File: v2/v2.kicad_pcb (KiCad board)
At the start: 2 copper layers, 9.7 x 8.4 mm, 97 parts, among them SW1 SW_Push, SW10 SW_Push, SW11 SW_Push, SW12 SW_Push, SW13 SW_Push, SW14 SW_Push, SW15 SW_Push, SW16 SW_Push, SW17 SW_Push, SW18 SW_Push, SW19 SW_Push, SW2 SW_Push, SW20 SW_Push, SW21 SW_Push, SW22 SW_Push, SW23 SW_Push, SW24 SW_Push, SW25 SW_Push, SW26 SW_Push, SW27 SW_Push, SW28 SW_Push, SW29 SW_Push, SW3 SW_Push, SW30 SW_Push, SW31 SW_Push, SW32 SW_Push, SW4 SW_Push, SW5 SW_Push, SW6 SW_Push, SW7 SW_Push, SW8 SW_Push, SW9 SW_Push, U1 Pico

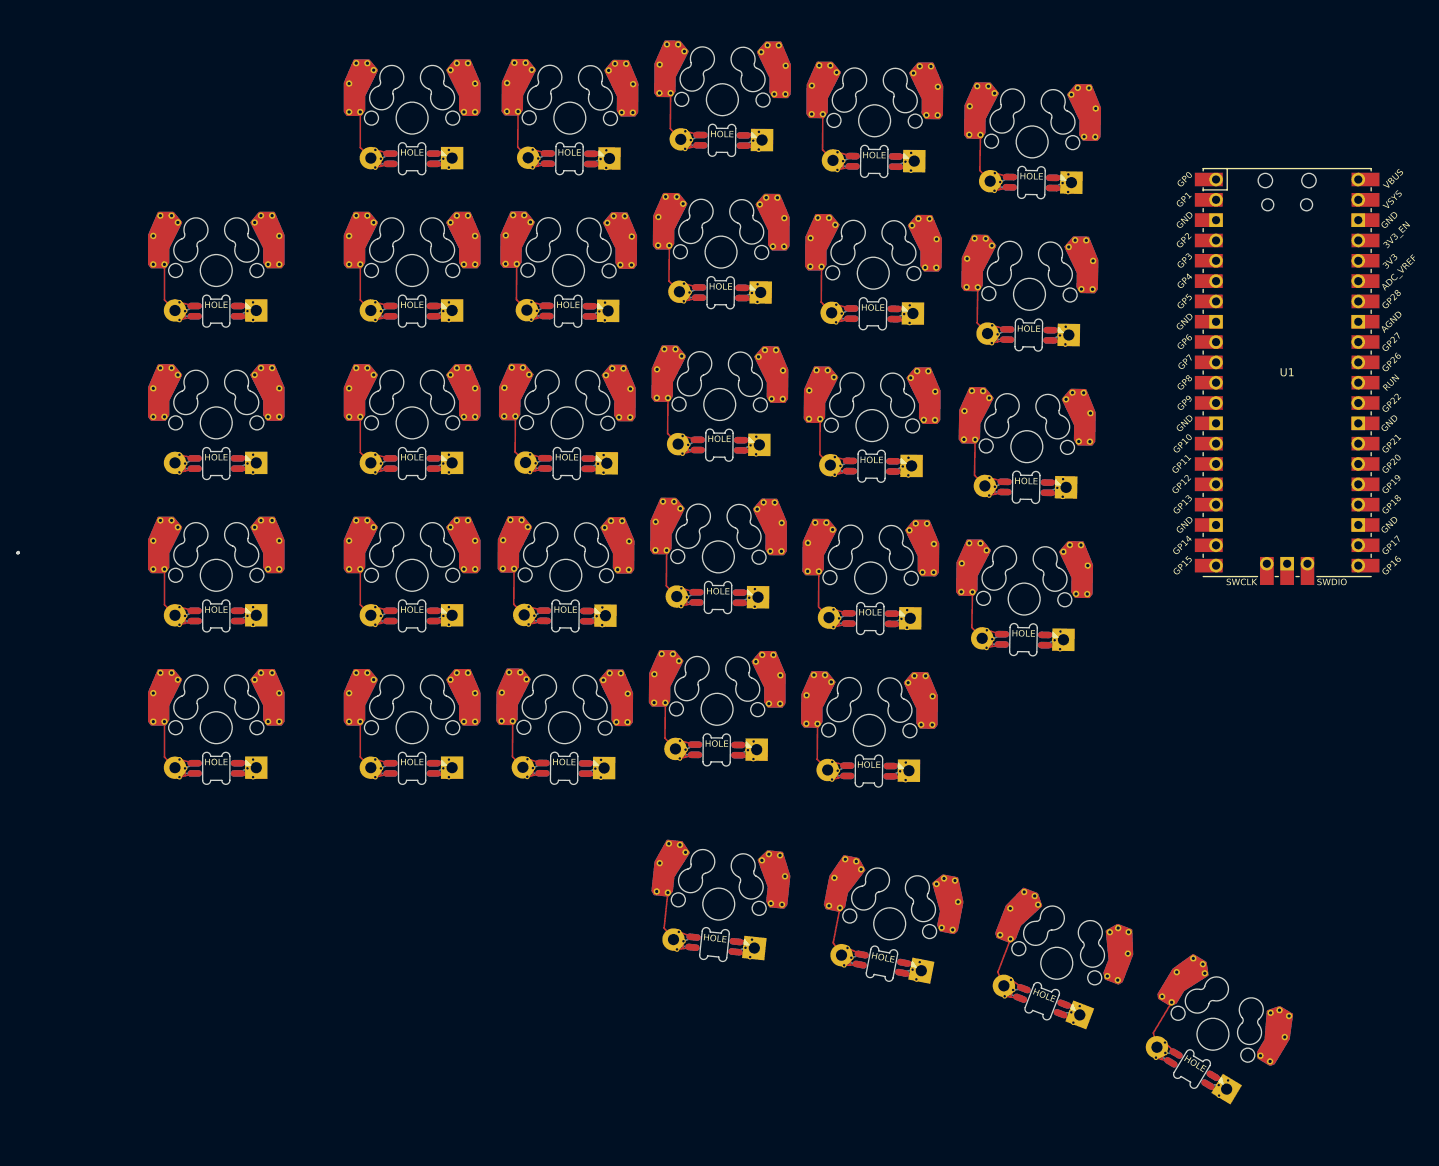
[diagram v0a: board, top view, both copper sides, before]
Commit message: schematic finished + some pcb
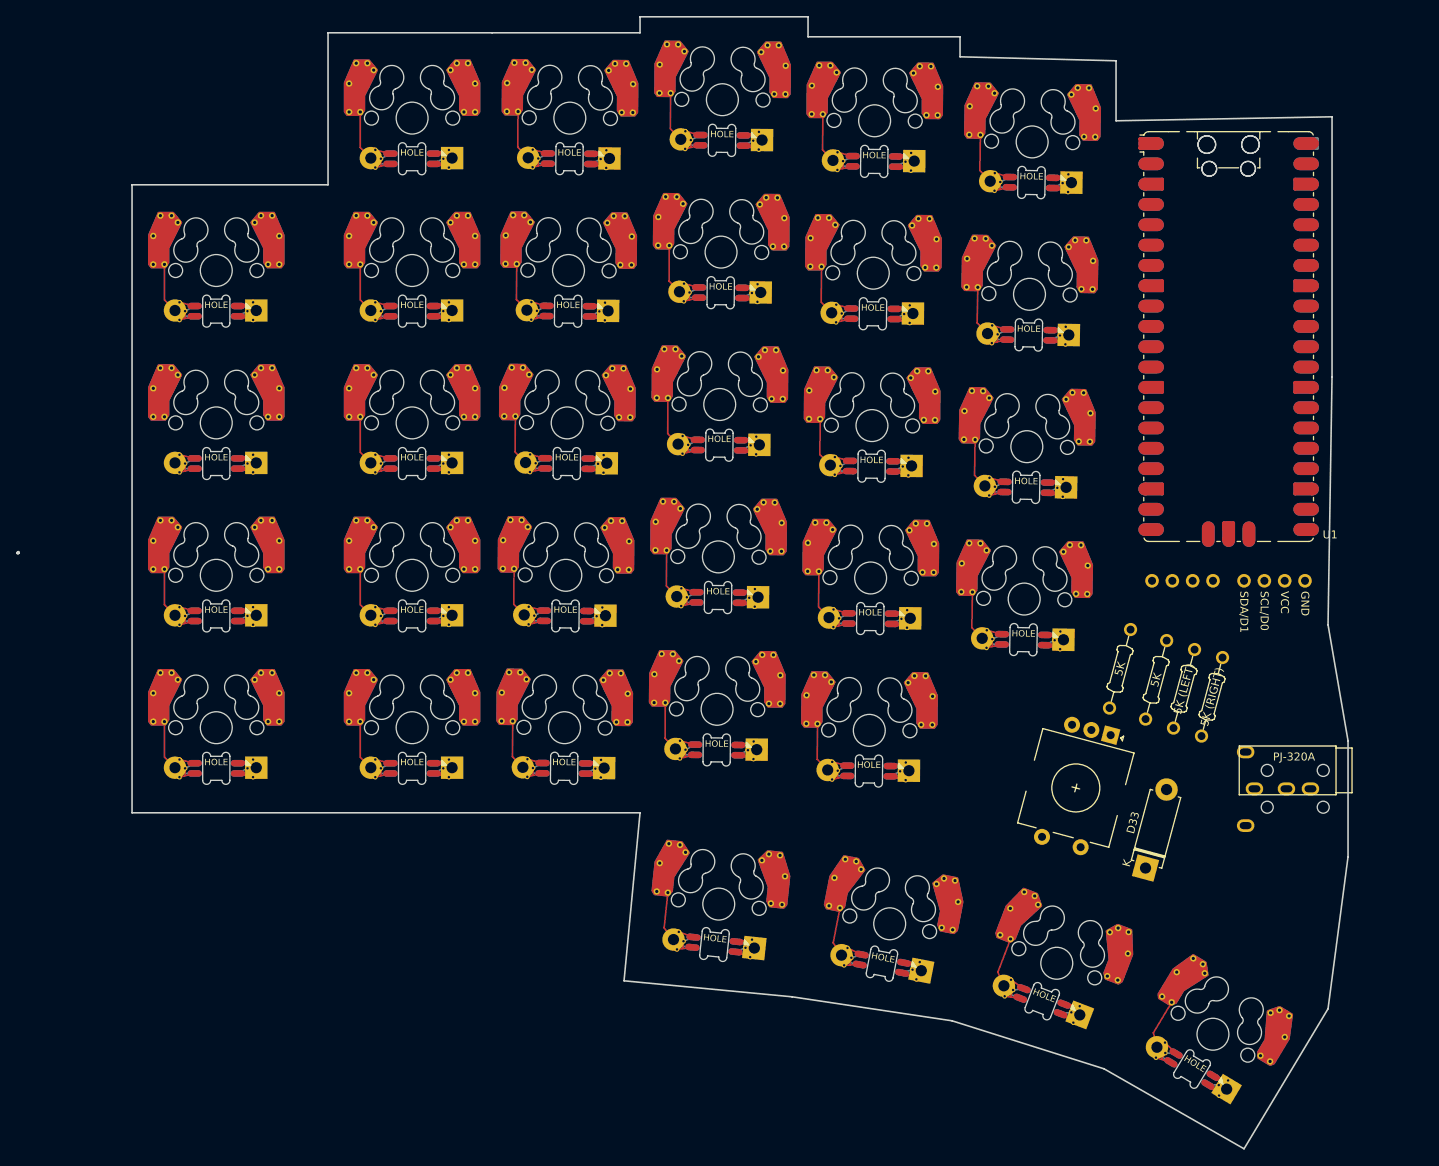
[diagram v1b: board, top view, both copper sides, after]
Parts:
- added D33: D, Diode_THT:D_5W_P10.16mm_Horizontal, F.Cu at (224.7, 186.4)
- added J1: Conn_01x04_Pin, Keebio-Parts:I2C_Breakout, F.Cu at (244.6, 150.5)
- added J2: Conn_01x04_Pin, Keebio-Parts:I2C_Breakout, B.Cu at (225.5, 150.5)
- added J3: Conn_01x04_Pin, Keebio-Parts:TRRS-PJ-320A-dual, F.Cu at (248.5, 176.5)
- added R1: 5K, Keebio-Parts:Resistor, F.Cu at (226.0, 162.9)
- added R2: 5K, Keebio-Parts:Resistor, F.Cu at (221.5, 161.5)
- added R3: 5K (LEFT), Keebio-Parts:Resistor, F.Cu at (229.5, 164.0)
- added R4: 5K (RIGHT), Keebio-Parts:Resistor, F.Cu at (233.0, 165.0)
- added SW33: RotaryEncoder_Switch, Keebio-Parts:RotaryEncoder_EC11, F.Cu at (216.0, 176.4)
- added U2: Pico, Module:RaspberryPi_Pico_SMD_HandSolder, B.Cu at (235.1, 120.0)
- U1: footprint RPi_Pico:RPi_Pico_SMD_TH -> Module:RaspberryPi_Pico_SMD_HandSolder
- moved U1 8.59 mm to (235.1, 120.0)
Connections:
- D29 pad 1: Net-(D29-K) -> Row 5
- D30 pad 1: Net-(D29-K) -> Row 5
- D31 pad 1: Net-(D29-K) -> Row 5
- D32 pad 1: Net-(D29-K) -> Row 5
- LED1 pad 3: unconnected-(LED1-DIN-Pad3) -> SK6912PWM
- U1 pad 1: unconnected-(U1-GPIO0-Pad1) -> Col 1
- U1 pad 10: unconnected-(U1-GPIO7-Pad10) -> Row 1
- U1 pad 11: unconnected-(U1-GPIO8-Pad11) -> Row 2
- U1 pad 12: unconnected-(U1-GPIO9-Pad12) -> Row 3
- U1 pad 13: unconnected-(U1-GND-Pad13) -> Row 4
- U1 pad 14: unconnected-(U1-GPIO10-Pad14) -> Row 5
- U1 pad 2: unconnected-(U1-GPIO1-Pad2) -> Col 2
- U1 pad 21: unconnected-(U1-GPIO16-Pad21) -> SPLIT SELECT
- U1 pad 24: unconnected-(U1-GPIO18-Pad24) -> SERIAL B
- U1 pad 25: unconnected-(U1-GPIO19-Pad25) -> SERIAL A
- U1 pad 39: unconnected-(U1-VSYS-Pad39) -> VSYS
- U1 pad 4: unconnected-(U1-GPIO2-Pad4) -> Col 3
- U1 pad 5: unconnected-(U1-GPIO3-Pad5) -> Col 4
- U1 pad 6: unconnected-(U1-GPIO4-Pad6) -> Col 5
- U1 pad 7: unconnected-(U1-GPIO5-Pad7) -> Col 6
- U1 pad 9: unconnected-(U1-GPIO6-Pad9) -> Col 7
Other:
- board size 9.7 x 8.4 mm -> 166.3 x 141.5 mm
